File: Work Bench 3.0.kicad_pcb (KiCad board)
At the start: 2 copper layers, 136 parts, among them J1 GND(A), J10 Lights 1 GND, J11 USB_A_Stacked, J12 Lights 2 GND, J13 Conn_01x02_Pin, J14 Lights 5V+(B), J15 Lights 1 GND, J16 Lights +5V(B), J17 Controls, J18 Lights 3 GND, J19 USB_A_Stacked, J2 GND(B), J20 Lights 4 GND, J21 Lights 4 GND, J22 Display, J23 Lights +5V(c), J24 Lights +5V(C), J25 Lights 3 GND, J26 Lights 5 GND, J27 Screw_Terminal_01x04, J28 Lights 6 GND, J29 Controls, J3 GND(C), J30 Lights 6 GND, J31 Lights +12V, J32 Lights +12V, J33 Lights 5 GND, J34 Extractor 1, J35 Extractor 2, J36 Extractor 3, J4 GND(12V), J5 +5V(A), J6 +5V(B), J7 +5V(C), J8 +12V, J9 Lights 2 GND, Q1 PMV20XNEAR, Q2 PMV20XNEAR, Q3 PMV20XNEAR, Q4 PMV20XNEAR, Q5 PMV20XNEAR, Q6 PMV20XNEAR, Q7 PMV20XNER, Q8 A2SHB, SW1 FSM4JSMA, SW2 FSM4JSMA, SW3 RotaryEncoder_Switch, U1 BCP5610TA, U10 BCP5610TA, U11 BCP53TA, U12 BCP5610TA, U13 BCP53TA, U2 BCP53TA, U3 Pico, U4 BCP5610TA, U5 BCP53TA, U6 BCP5610TA, U7 BCP53TA, U8 BCP5610TA, U9 BCP53TA

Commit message: Done
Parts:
- removed J15: Lights 1 GND, Connector_Wire:SolderWirePad_1x01_SMD_5x10mm
- removed J16: Lights +5V(B), Connector_Wire:SolderWirePad_1x01_SMD_5x10mm
- removed J18, J25: Lights 3 GND, Connector_Wire:SolderWirePad_1x01_SMD_5x10mm
- removed J20, J21: Lights 4 GND, Connector_Wire:SolderWirePad_1x01_SMD_5x10mm
- removed J23: Lights +5V(c), Connector_Wire:SolderWirePad_1x01_SMD_5x10mm
- removed J24: Lights +5V(C), Connector_Wire:SolderWirePad_1x01_SMD_5x10mm
- removed J26, J33: Lights 5 GND, Connector_Wire:SolderWirePad_1x01_SMD_5x10mm
- removed J28, J30: Lights 6 GND, Connector_Wire:SolderWirePad_1x01_SMD_5x10mm
- removed J31, J32: Lights +12V, Connector_Wire:SolderWirePad_1x01_SMD_5x10mm
- added J37: Conn_01x04_Pin, SMD-Connectors:SMD-PinHeader_1x04_P2.54mm_Vertical, F.Cu at (84.3, 35.8)
- added J38: 5V Lights, SMD-Connectors:SMD-PinHeader_1x04_P2.54mm_Vertical, F.Cu at (183.2, 60.5)
- J10: value Lights 1 GND -> Conn_01x02_Pin; footprint Connector_Wire:SolderWirePad_1x01_SMD_5x10mm -> SMD-Connectors:SMD-PinHeader_1x02_P2.54mm_Vertical
- J12: value Lights 2 GND -> GND(12V)
- J14: value Lights 5V+(B) -> +12V
- J9: value Lights 2 GND -> Conn_01x02_Pin; footprint Connector_Wire:SolderWirePad_1x01_SMD_5x10mm -> SMD-Connectors:SMD-PinHeader_1x02_P2.54mm_Vertical
- moved J14 216.4 mm to (243.8, 40.2)
- moved J12 206.4 mm to (236.2, 40.2)
- moved J10 150.0 mm to (183.2, 83.3)
- moved J9 97.6 mm to (132.8, 36.7), turned to 180 degrees
- moved C31 96.5 mm to (110.8, 180.1)
- moved J29 96.5 mm to (71.1, 138.4)
- moved R21 96.5 mm to (110.8, 142.1)
- moved R24 96.5 mm to (102.6, 184.5)
- moved SW1 96.5 mm to (56.0, 159.7)
- moved SW2 96.5 mm to (56.0, 167.3)
- moved SW3 96.5 mm to (104.2, 170.7)
- moved C18 96.5 mm to (49.8, 152.2)
- moved C23 96.5 mm to (49.8, 174.8)
- moved C28 96.5 mm to (102.6, 180.1)
- moved C29 96.5 mm to (110.8, 146.1)
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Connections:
- C13 pad 1: Net-(J19-VBUS1) -> +5V(C)
- C13 pad 2: Net-(J18-Pin_1) -> Net-(J19-GND1)
- C14 pad 1: Net-(J19-VBUS1) -> +5V(C)
- C22 pad 1: Net-(J27-Pin_2) -> +12V
- C22 pad 2: Net-(J26-Pin_1) -> Net-(J27-Pin_1)
- C24 pad 1: Net-(J27-Pin_2) -> +12V
- C6 pad 1: Net-(J11-VBUS1) -> +5V(B)
- C6 pad 2: Net-(J10-Pin_1) -> Net-(J11-GND1)
- C8 pad 1: Net-(J11-VBUS1) -> +5V(B)
- J11 pad 1: Net-(J11-VBUS1) -> +5V(B)
- J11 pad 4: Net-(J10-Pin_1) -> Net-(J11-GND1)
- J11 pad 5: Net-(J11-VBUS1) -> +5V(B)
- J12 pad 1: Net-(J11-GND2) -> GND
- J14 pad 1: +5V(B) -> +12V
- J19 pad 1: Net-(J19-VBUS1) -> +5V(C)
- J19 pad 4: Net-(J18-Pin_1) -> Net-(J19-GND1)
- J19 pad 5: Net-(J19-VBUS1) -> +5V(C)
- J27 pad 1: Net-(J26-Pin_1) -> Net-(J27-Pin_1)
- J27 pad 2: Net-(J27-Pin_2) -> +12V
- J27 pad 4: Net-(J27-Pin_2) -> +12V
- Q1 pad 3: Net-(J9-Pin_1) -> Net-(J11-GND2)
- Q2 pad 3: Net-(J15-Pin_1) -> Net-(J11-GND1)
- Q3 pad 3: Net-(J21-Pin_1) -> Net-(J19-GND2)
- Q4 pad 3: Net-(J25-Pin_1) -> Net-(J19-GND1)
- Q5 pad 3: Net-(J30-Pin_1) -> Net-(J27-Pin_3)
- Q6 pad 3: Net-(J33-Pin_1) -> Net-(J27-Pin_1)
- R10 pad 1: /Lights 4 Signal -> Net-(J37-Pin_4)
- R15 pad 1: /Lights 3 Signal -> Net-(J37-Pin_3)
- R2 pad 1: /Lights 2 Signal -> Net-(J37-Pin_2)
- R20 pad 1: /Lights 6 Signal -> Net-(J9-Pin_2)
- R26 pad 1: /Lights 5 Signal -> Net-(J9-Pin_1)
- R6 pad 1: /Lights 1 Signal -> Net-(J37-Pin_1)
- U3 pad 11: /Lights 4 Signal -> Net-(J38-Pin_4)
- U3 pad 14: /Lights 5 Signal -> Net-(J10-Pin_1)
- U3 pad 16: /Lights 6 Signal -> Net-(J10-Pin_2)
- U3 pad 4: /Lights 1 Signal -> Net-(J38-Pin_1)
- U3 pad 6: /Lights 2 Signal -> Net-(J38-Pin_2)
- U3 pad 9: /Lights 3 Signal -> Net-(J38-Pin_3)
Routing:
- net /Lights 1 Signal: track 133.1 -> 0.00 mm
- net /Lights 2 Signal: track 125.5 -> 0.00 mm
- net /Lights 3 Signal: track 106.1 -> 0.00 mm
- net /Lights 4 Signal: track 98.5 -> 0.00 mm
- net Net-(D1-A): track 115.8 -> 192.9 mm
- net Net-(J27-Pin_2): track 72.0 -> 0.00 mm
- net Net-(J37-Pin_2): track 0.00 -> 63.6 mm
- net /Lights 5 Signal: track 61.1 -> 0.00 mm
- net Net-(J37-Pin_1): track 0.00 -> 59.7 mm
- net /Lights 6 Signal: track 52.2 -> 0.00 mm
- net Net-(J18-Pin_1): track 43.9 -> 0.00 mm
- net +12V: track 359.7 -> 318.0 mm
- net Net-(J26-Pin_1): track 41.0 -> 0.00 mm
- net Net-(J11-GND1): track 0.00 -> 36.8 mm
- net Net-(J19-GND1): track 0.00 -> 36.7 mm
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- added copper zone on F.Cu, net Net-(J11-GND1)
- added copper zone on F.Cu, net Net-(J11-GND2)
- added copper zone on F.Cu, net Net-(J19-GND1)
- added copper zone on F.Cu, net Net-(J19-GND2)
- added copper zone on F.Cu, net Net-(J27-Pin_1)
- added copper zone on F.Cu, net Net-(J27-Pin_3)
- removed copper zone on F.Cu, net Net-(J15-Pin_1)
- removed copper zone on F.Cu, net Net-(J21-Pin_1)
- removed copper zone on F.Cu, net Net-(J25-Pin_1)
- removed copper zone on F.Cu, net Net-(J30-Pin_1)
- removed copper zone on F.Cu, net Net-(J33-Pin_1)
- removed copper zone on F.Cu, net Net-(J9-Pin_1)

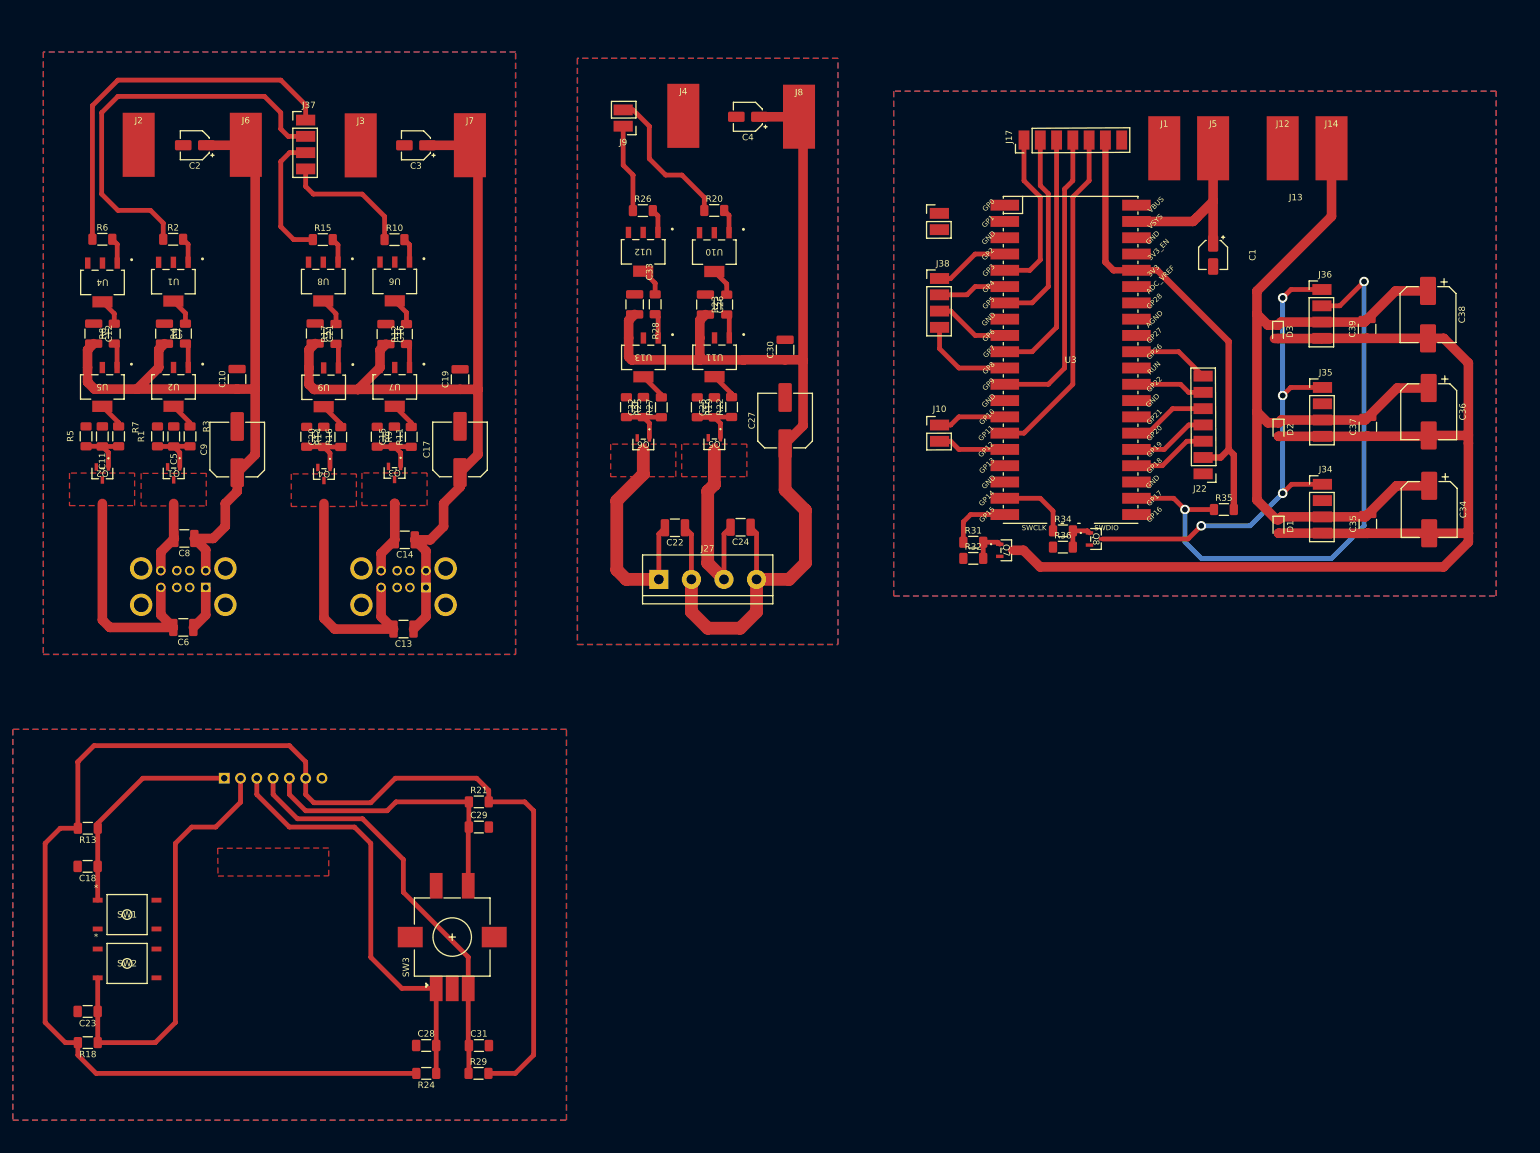
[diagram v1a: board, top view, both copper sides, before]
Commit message: Split
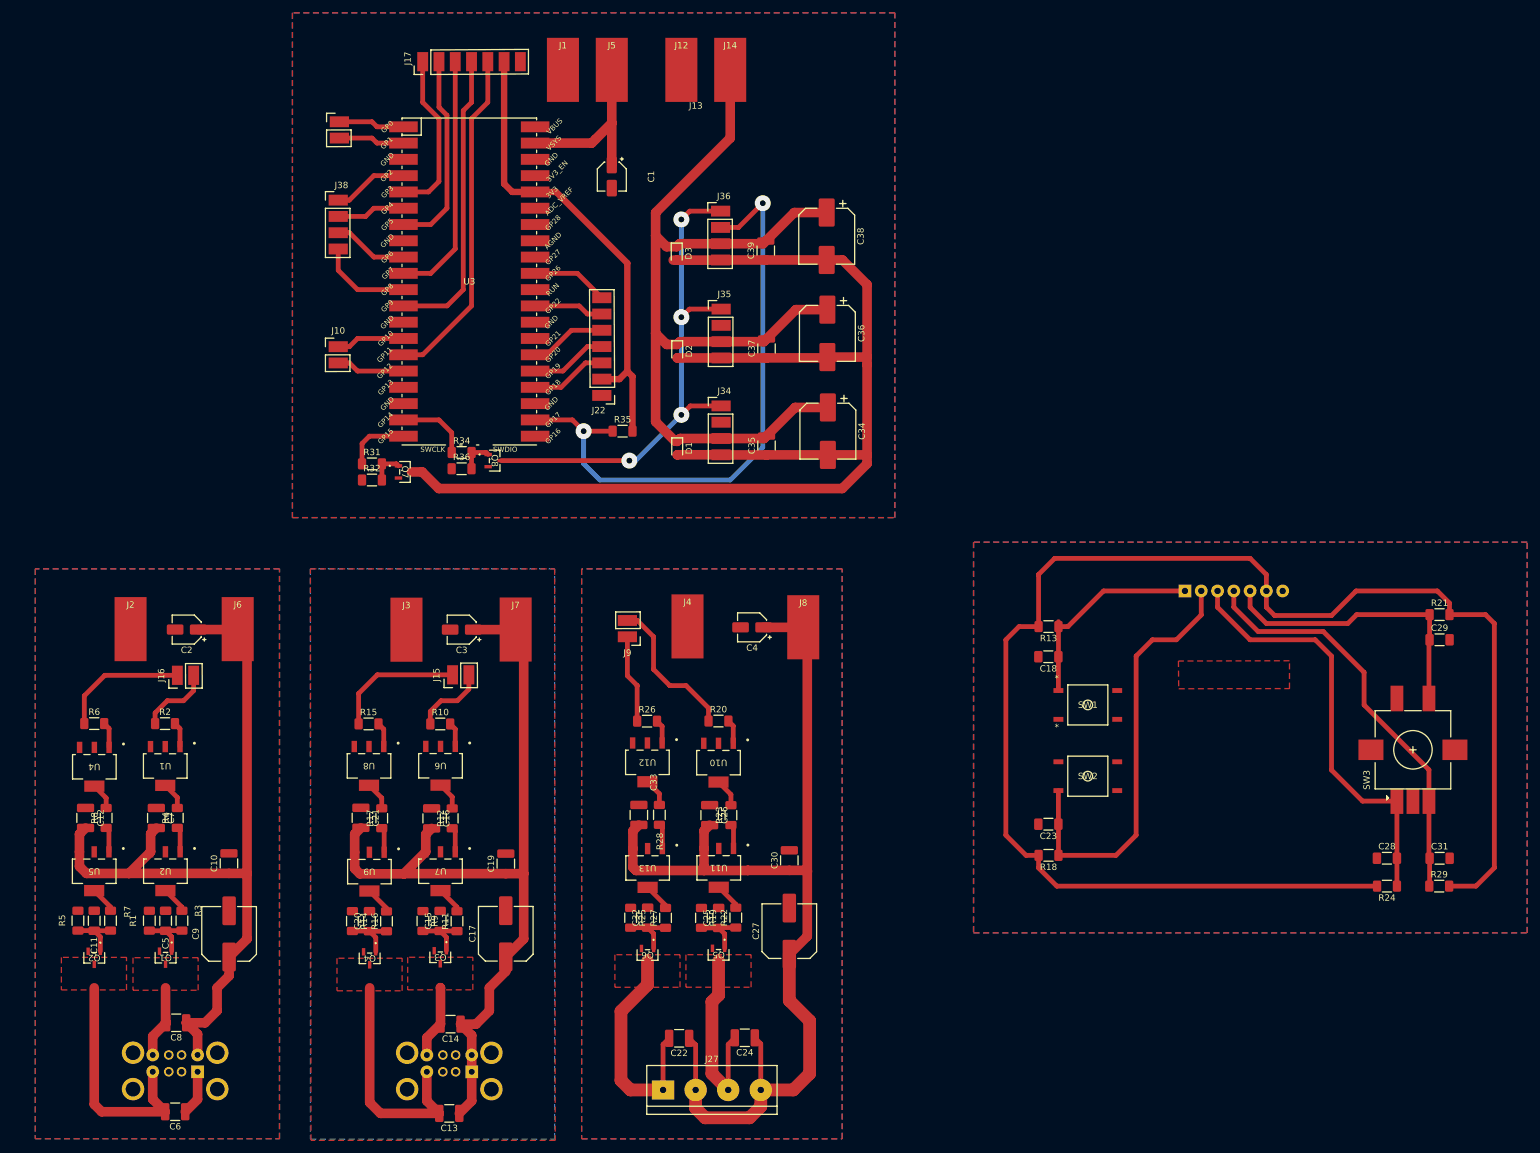
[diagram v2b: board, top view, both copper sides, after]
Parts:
- removed J37: Conn_01x04_Pin, SMD-Connectors:SMD-PinHeader_1x04_P2.54mm_Vertical
- added J15: Conn_01x02_Pin, SMD-Connectors:SMD-PinHeader_1x02_P2.54mm_Vertical, F.Cu at (106.7, 121.8)
- added J16: Conn_01x02_Pin, SMD-Connectors:SMD-PinHeader_1x02_P2.54mm_Vertical, F.Cu at (63.8, 121.9)
- moved C18 153.4 mm to (199.7, 119.5)
- moved SW1 153.4 mm to (205.8, 127.0)
- moved R13 153.1 mm to (199.7, 114.8)
- moved C23 152.7 mm to (199.7, 145.6)
- moved C28 152.7 mm to (252.5, 150.9)
- moved R18 152.7 mm to (199.7, 150.5)
- moved R24 152.7 mm to (252.5, 155.3)
- moved C31 152.7 mm to (260.7, 150.9)
- moved J29 152.7 mm to (221.0, 109.2)
- moved R21 152.7 mm to (260.7, 112.9)
- moved SW2 152.7 mm to (205.8, 138.1)
- moved SW3 152.7 mm to (254.0, 141.5)
- moved C29 152.7 mm to (260.7, 116.8)
- moved R29 152.7 mm to (260.6, 155.3)
- moved J13 94.7 mm to (89.6, 36.0)
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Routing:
- net Net-(J16-Pin_2): track 63.6 -> 11.5 mm
- net Net-(J16-Pin_1): track 59.7 -> 20.2 mm
- net Net-(J13-Pin_2): track 0.00 -> 11.7 mm
- net Net-(J13-Pin_1): track 0.00 -> 11.7 mm
- net Net-(J15-Pin_2): track 20.6 -> 11.7 mm
- net +12V: track 318.0 -> 312.6 mm
- net Net-(J29-Pin_1): track 34.6 -> 32.8 mm
